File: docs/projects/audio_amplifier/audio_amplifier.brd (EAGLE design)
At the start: 39 x 48.2 mm, 23 parts, among them IC1 UA741P, IC2 LM386N-1

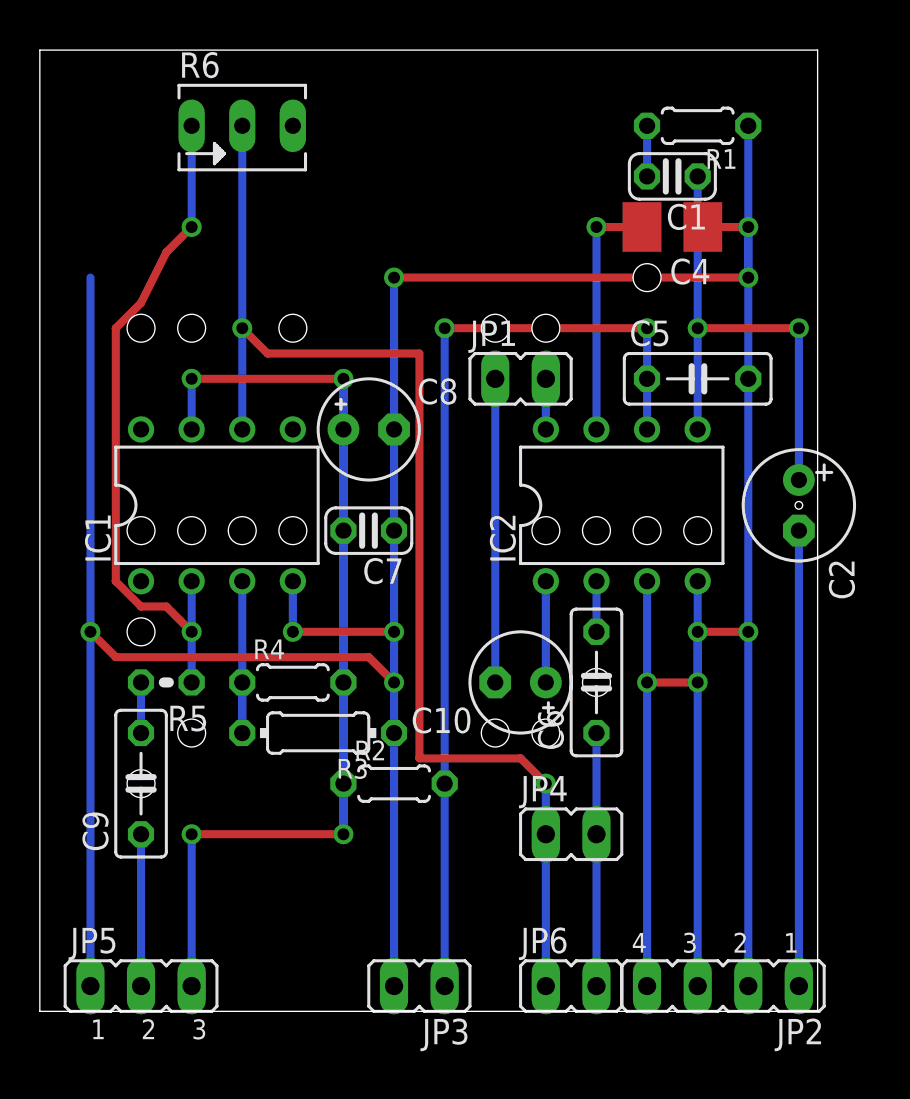
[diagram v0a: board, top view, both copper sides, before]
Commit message: fix airwires
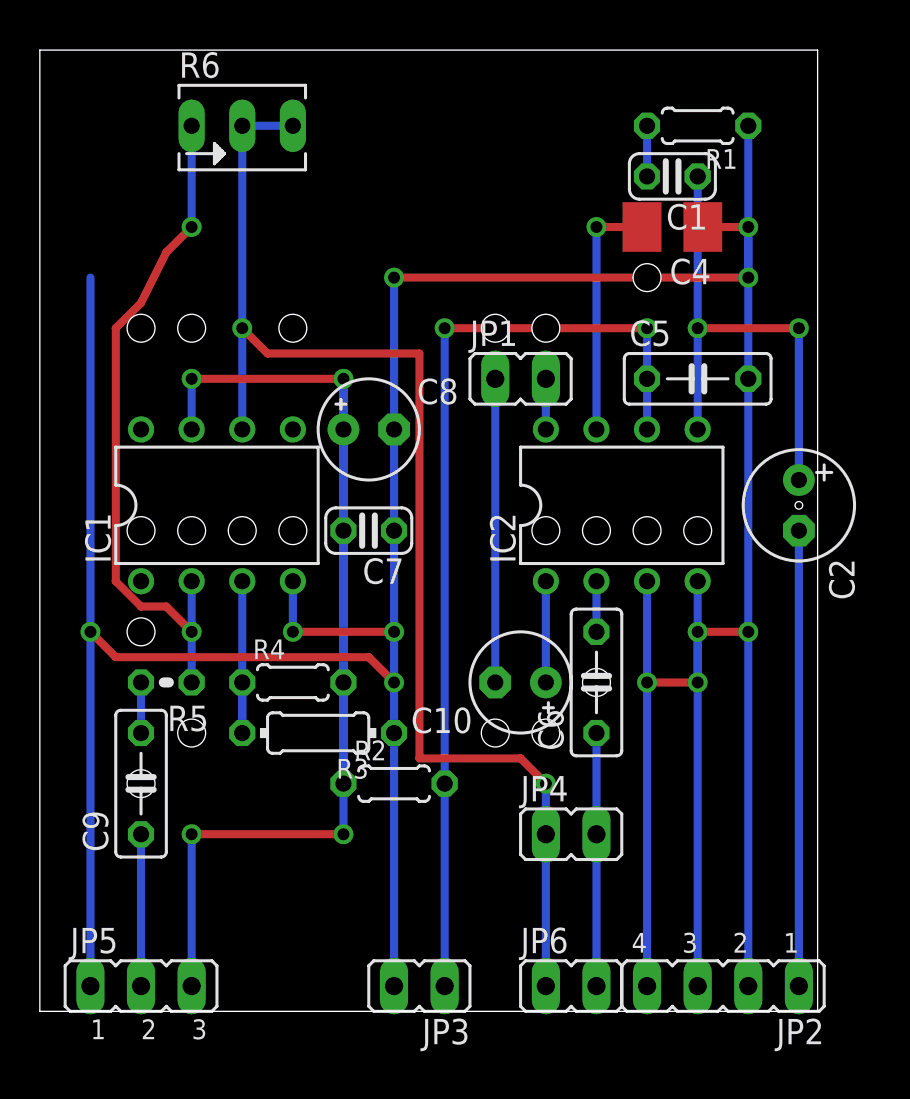
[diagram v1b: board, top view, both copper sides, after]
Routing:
- net N$7: track 86.4 -> 81.3 mm
- net N$15: track 62.0 -> 64.6 mm
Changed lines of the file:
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@@
 <wire x1="22.86" y1="17.78" x2="22.86" y2="20.32" width="0.4064" layer="16"/>
 <wire x1="22.86" y1="17.78" x2="22.86" y2="15.24" width="0.4064" layer="16"/>
-<wire x1="22.86" y1="20.32" x2="22.86" y2="30.48" width="0.4064" layer="16"/>
+<wire x1="22.86" y1="20.32" x2="22.86" y2="25.4" width="0.4064" layer="16"/>
 <wire x1="22.86" y1="20.32" x2="17.78" y2="20.32" width="0.4064" layer="1"/>
 <wire x1="7.62" y1="20.32" x2="8.89" y2="19.05" width="0.4064" layer="1"/>
@@
 <wire x1="38.1" y1="17.78" x2="38.1" y2="2.54" width="0.4064" layer="16"/>
 <wire x1="35.56" y1="17.78" x2="35.56" y2="2.54" width="0.4064" layer="16"/>
-<wire x1="22.86" y1="30.48" x2="22.86" y2="25.4" width="0" layer="19" extent="16-16"/>
 <via x="17.78" y="20.32" extent="1-16" drill="0.6" shape="square"/>
 <via x="40.64" y="20.32" extent="1-16" drill="0.6" shape="square"/>
@@
 <via x="22.86" y="20.32" extent="1-16" drill="0.6" shape="square"/>
 <via x="22.86" y="17.78" extent="1-16" drill="0.6" shape="square"/>
+<wire x1="22.86" y1="30.48" x2="22.86" y2="25.4" width="0.4064" layer="16"/>
 </signal>
 <signal name="N$2">
@@
 <contactref element="C8" pad="+"/>
 <contactref element="JP5" pad="3"/>
-<wire x1="20.32" y1="10.16" x2="20.32" y2="17.78" width="0.4064" layer="16"/>
-<wire x1="20.32" y1="10.16" x2="20.32" y2="30.48" width="0.4064" layer="16"/>
+<wire x1="20.32" y1="12.7" x2="20.32" y2="17.78" width="0.4064" layer="16"/>
+<wire x1="20.32" y1="12.7" x2="20.32" y2="30.48" width="0.4064" layer="16"/>
 <wire x1="12.7" y1="33.02" x2="12.7" y2="30.48" width="0.4064" layer="16"/>
 <wire x1="20.32" y1="30.48" x2="20.32" y2="33.02" width="0.4064" layer="16"/>
 <wire x1="20.32" y1="33.02" x2="12.7" y2="33.02" width="0.4064" layer="1"/>
-<wire x1="20.32" y1="10.16" x2="20.32" y2="33.02" width="0.4064" layer="16"/>
+<wire x1="20.32" y1="12.7" x2="20.32" y2="33.02" width="0.4064" layer="16"/>
 <wire x1="12.7" y1="2.54" x2="12.7" y2="10.16" width="0.4064" layer="16"/>
 <wire x1="12.7" y1="10.16" x2="20.32" y2="10.16" width="0.4064" layer="1"/>
 <wire x1="20.32" y1="33.02" x2="20.32" y2="25.4" width="0.4064" layer="16"/>
-<wire x1="20.32" y1="10.16" x2="20.32" y2="12.7" width="0" layer="19" extent="16-16"/>
 <via x="12.7" y="33.02" extent="1-16" drill="0.6" shape="square"/>
 <via x="20.32" y="33.02" extent="1-16" drill="0.6" shape="square"/>
 <via x="20.32" y="10.16" extent="1-16" drill="0.6" shape="square"/>
 <via x="12.7" y="10.16" extent="1-16" drill="0.6" shape="square"/>
+<wire x1="20.32" y1="10.16" x2="20.32" y2="12.7" width="0.4064" layer="16"/>
 </signal>
 <signal name="N$8">
@@
 <wire x1="24.13" y1="13.97" x2="24.13" y2="34.29" width="0.4064" layer="1"/>
 <wire x1="30.48" y1="2.54" x2="30.48" y2="10.16" width="0.4064" layer="16"/>
-<wire x1="15.24" y1="45.72" x2="17.78" y2="45.72" width="0" layer="19" extent="1-1"/>
 <via x="30.48" y="12.7" extent="1-16" drill="0.6" shape="square"/>
 <via x="15.24" y="35.56" extent="1-16" drill="0.6" shape="square"/>
+<wire x1="15.24" y1="45.72" x2="17.78" y2="45.72" width="0.4064" layer="16"/>
 </signal>
 <signal name="N$17">
